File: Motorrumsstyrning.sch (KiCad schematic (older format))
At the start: 49 parts, among them J1 Jumper, J10 Jumper, J11 Jumper, J12 SD_Card_Connector, J13 Jumper, J14 Conn_01x09, J15 Screw_Terminal_01x10, J2 Jumper, J3 Jumper, J4 Jumper, J5 Screw_Terminal_01x10, J6 Jumper, J7 Jumper, J8 Jumper, J9 Jumper, Q1 BC337, Q2 BC337, U1 LM1084-5.0, U2 MCP2551-I-P, U3 NUCLEO-F303K8

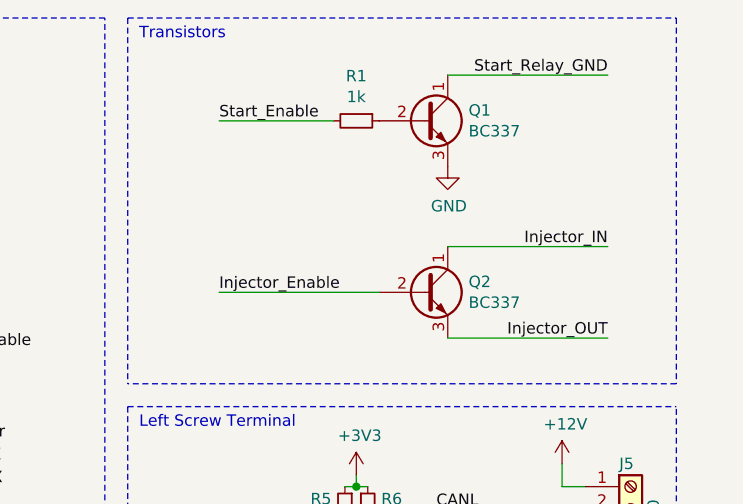
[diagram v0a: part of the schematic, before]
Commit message: Update
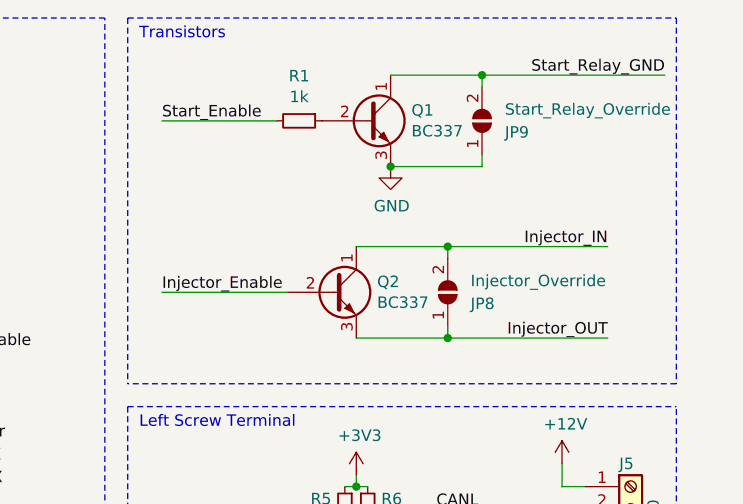
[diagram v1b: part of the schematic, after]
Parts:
- added JP8: Injector_Override, Jumper:SolderJumper-2_P1.3mm_Open_TrianglePad1.0x1.5mm, symbol Jumper:SolderJumper_2_Open
- added JP9: Start_Relay_Override, Jumper:SolderJumper-2_P1.3mm_Open_TrianglePad1.0x1.5mm, symbol Jumper:SolderJumper_2_Open
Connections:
- net GND: now also JP9.1 (A)
- net Injector_IN: now also JP8.2 (B)
- net Injector_OUT: now also JP8.1 (A)
- net Start_Relay_GND: now also JP9.2 (B)
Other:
- moved on the sheet: Q1, Q2, R1
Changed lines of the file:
@@
 L Transistor_BJT:BC337 Q1
 U 1 1 60C819FD
-P 10050 1000
-F 0 "Q1" H 10241 1046 50  0000 L CNN
-F 1 "BC337" H 10241 955 50  0000 L CNN
-F 2 "Package_TO_SOT_THT:TO-92_Inline" H 10250 925 50  0001 L CIN
-F 3 "https://diotec.com/tl_files/diotec/files/pdf/datasheets/bc337.pdf" H 10050 1000 50  0001 L CNN
-	1    10050 1000
-	1    0    0    -1
-$EndComp
-Text Label 10850 800  2    50   ~ 0
+P 9800 1000
+F 0 "Q1" H 9991 1046 50  0000 L CNN
+F 1 "BC337" H 9991 955 50  0000 L CNN
+F 2 "Package_TO_SOT_THT:TO-92_Inline" H 10000 925 50  0001 L CIN
+F 3 "https://diotec.com/tl_files/diotec/files/pdf/datasheets/bc337.pdf" H 9800 1000 50  0001 L CNN
+	1    9800 1000
+	1    0    0    -1
+$EndComp
+Text Label 11100 800  2    50   ~ 0
 Start_Relay_GND
 $Comp
 L power:GND #PWR06
 U 1 1 60C82964
-P 10150 1200
-F 0 "#PWR06" H 10150 950 50  0001 C CNN
-F 1 "GND" H 10155 1027 50  0000 C CNN
-F 2 "" H 10150 1200 50  0001 C CNN
-F 3 "" H 10150 1200 50  0001 C CNN
-	1    10150 1200
+P 9900 1200
+F 0 "#PWR06" H 9900 950 50  0001 C CNN
+F 1 "GND" H 9905 1027 50  0000 C CNN
+F 2 "" H 9900 1200 50  0001 C CNN
+F 3 "" H 9900 1200 50  0001 C CNN
+	1    9900 1200
 	1    0    0    -1
 $EndComp
@@
 L Device:R_Small R1
 U 1 1 60C832BB
-P 9750 1000
-F 0 "R1" V 9554 1000 50  0000 C CNN
-F 1 "1k" V 9645 1000 50  0000 C CNN
-F 2 "Resistor_THT:R_Axial_DIN0207_L6.3mm_D2.5mm_P7.62mm_Horizontal" H 9750 1000 50  0001 C CNN
-F 3 "~" H 9750 1000 50  0001 C CNN
-	1    9750 1000
+P 9500 1000
+F 0 "R1" V 9304 1000 50  0000 C CNN
+F 1 "1k" V 9395 1000 50  0000 C CNN
+F 2 "Resistor_THT:R_Axial_DIN0207_L6.3mm_D2.5mm_P7.62mm_Horizontal" H 9500 1000 50  0001 C CNN
+F 3 "~" H 9500 1000 50  0001 C CNN
+	1    9500 1000
 	0    1    1    0
 $EndComp
-Text Label 9150 1000 0    50   ~ 0
+Text Label 8900 1000 0    50   ~ 0
 Start_Enable
 Wire Wire Line
-	9650 1000 9150 1000
+	9400 1000 8900 1000
 Text Label 10850 1550 2    50   ~ 0
 Injector_IN
@@
 L Transistor_BJT:BC337 Q2
 U 1 1 60C8DD08
-P 10050 1750
-F 0 "Q2" H 10241 1796 50  0000 L CNN
-F 1 "BC337" H 10241 1705 50  0000 L CNN
-F 2 "Package_TO_SOT_THT:TO-92_Inline" H 10250 1675 50  0001 L CIN
-F 3 "https://diotec.com/tl_files/diotec/files/pdf/datasheets/bc337.pdf" H 10050 1750 50  0001 L CNN
-	1    10050 1750
+P 9650 1750
+F 0 "Q2" H 9841 1796 50  0000 L CNN
+F 1 "BC337" H 9841 1705 50  0000 L CNN
+F 2 "Package_TO_SOT_THT:TO-92_Inline" H 9850 1675 50  0001 L CIN
+F 3 "https://diotec.com/tl_files/diotec/files/pdf/datasheets/bc337.pdf" H 9650 1750 50  0001 L CNN
+	1    9650 1750
 	1    0    0    -1
 $EndComp
@@
 	10850 1950 10150 1950
 Wire Wire Line
-	10150 1550 10850 1550
+	9750 1550 10150 1550
 Text Label 7800 2000 0    50   ~ 0
 Injector_Enable
-Text Label 9150 1750 0    50   ~ 0
+Text Label 8900 1750 0    50   ~ 0
 Injector_Enable
 Wire Wire Line
-	9150 1750 9850 1750
+	8900 1750 9450 1750
 Text Label 7800 1900 0    50   ~ 0
 PA3
@@
 Text Notes 8800 2350 0    50   ~ 0
 Left Screw Terminal
-Wire Wire Line
-	10150 800  10850 800
 Wire Notes Line
 	11150 2150 8750 2150
@@
 	1    0    0    -1
 $EndComp
+$Comp
+L Jumper:SolderJumper_2_Open JP9
+U 1 1 613A7272
+P 10300 1000
+F 0 "JP9" V 10250 1100 50  0000 L CNN
+F 1 "Start_Relay_Override" V 10350 1100 50  0000 L CNN
+F 2 "Jumper:SolderJumper-2_P1.3mm_Open_TrianglePad1.0x1.5mm" H 10300 1000 50  0001 C CNN
+F 3 "~" H 10300 1000 50  0001 C CNN
+	1    10300 1000
+	0    1    -1   0
+$EndComp
+$Comp
+L Jumper:SolderJumper_2_Open JP8
+U 1 1 613B8773
+P 10150 1750
+F 0 "JP8" V 10100 1850 50  0000 L CNN
+F 1 "Injector_Override" V 10200 1850 50  0000 L CNN
+F 2 "Jumper:SolderJumper-2_P1.3mm_Open_TrianglePad1.0x1.5mm" H 10150 1750 50  0001 C CNN
+F 3 "~" H 10150 1750 50  0001 C CNN
+	1    10150 1750
+	0    1    -1   0
+$EndComp
+Wire Wire Line
+	10150 1600 10150 1550
+Connection ~ 10150 1550
+Wire Wire Line
+	10150 1550 10850 1550
+Wire Wire Line
+	10150 1900 10150 1950
+Connection ~ 10150 1950
+Wire Wire Line
+	10150 1950 9750 1950
+Wire Wire Line
+	9900 800  10300 800
+Wire Wire Line
+	10300 850  10300 800
+Connection ~ 10300 800
+Wire Wire Line
+	10300 800  11100 800
+Wire Wire Line
+	10300 1150 10300 1200
+Wire Wire Line
+	10300 1200 9900 1200
+Connection ~ 9900 1200
 $EndSCHEMATC
